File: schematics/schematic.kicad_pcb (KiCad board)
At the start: 2 copper layers, 79.5 x 90 mm, 6 parts, among them Q1 BPW40, U1 L293D, U2 ESP32-S3-DevKitC

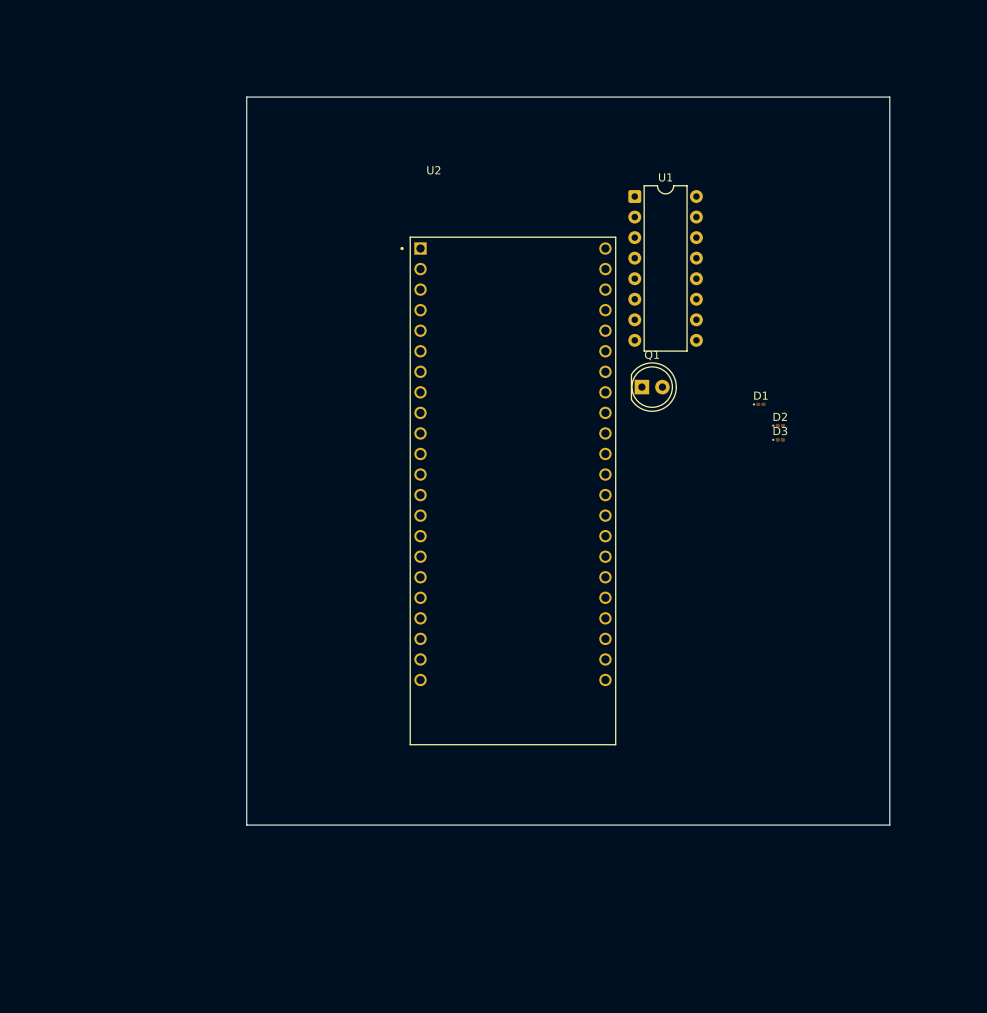
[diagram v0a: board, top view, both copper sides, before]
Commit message: schematic updates
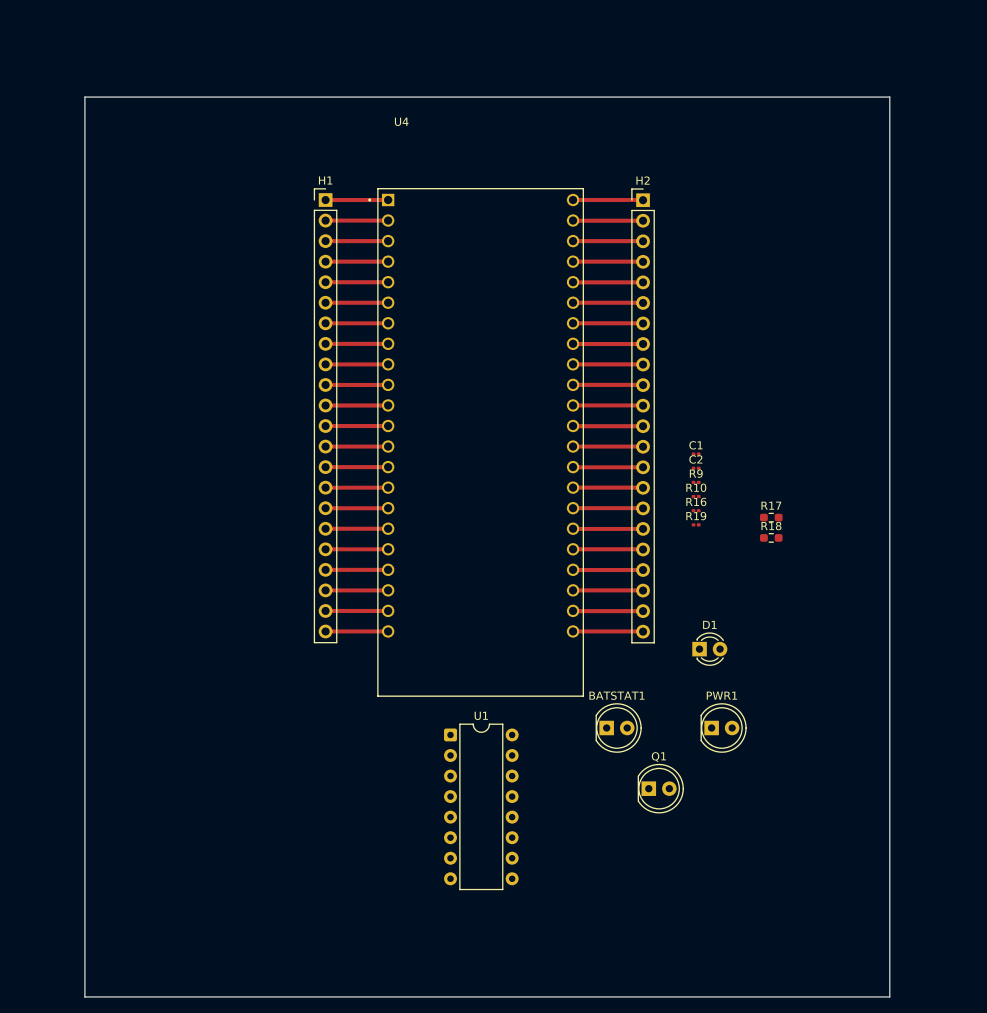
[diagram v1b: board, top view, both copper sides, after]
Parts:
- removed D2: GREEN, LED_SMD:LED_0201_0603Metric
- removed D3: BLUE, LED_SMD:LED_0201_0603Metric
- removed U2: ESP32-S3-DevKitC, footprints_pretty:XCVR_ESP32-S3-DEVKITC-1-N8R2
- added BATSTAT1: LED, LED_THT:LED_D5.0mm, F.Cu at (165.2, 127.5)
- added C1: 0.33 uF, Capacitor_SMD:C_0201_0603Metric, F.Cu at (176.3, 93.6)
- added C2: 0.1 uF, Capacitor_SMD:C_0201_0603Metric, F.Cu at (176.3, 95.4)
- added H1: ~, Connector_PinHeader_2.54mm:PinHeader_1x22_P2.54mm_Vertical, F.Cu at (130.5, 62.2)
- added H2: ~, Connector_PinHeader_2.54mm:PinHeader_1x22_P2.54mm_Vertical, F.Cu at (169.8, 62.2)
- added PWR1: LED, LED_THT:LED_D5.0mm, F.Cu at (178.2, 127.5)
- added R10: 110 kΩ, Resistor_SMD:R_0201_0603Metric, F.Cu at (176.3, 98.9)
- added R16: 1.5 kΩ, Resistor_SMD:R_0201_0603Metric, F.Cu at (176.3, 100.6)
- added R17: 4.7 MΩ, Resistor_SMD:R_0603_1608Metric_Pad0.98x0.95mm_HandSolder, F.Cu at (185.6, 101.5)
- added R18: 2.56 MΩ, Resistor_SMD:R_0603_1608Metric_Pad0.98x0.95mm_HandSolder, F.Cu at (185.6, 104.0)
- added R19: 1.5 kΩ, Resistor_SMD:R_0201_0603Metric, F.Cu at (176.3, 102.4)
- added R9: 110 Ω, Resistor_SMD:R_0201_0603Metric, F.Cu at (176.3, 97.1)
- added U4: ESP32-S3-DEVKITC-1-N8R2, footprints_pretty:XCVR_ESP32-S3-DEVKITC-1-N8R2, F.Cu at (149.7, 92.2)
- D1: value RED -> IR204A; footprint LED_SMD:LED_0201_0603Metric -> LED_THT:LED_D3.0mm_IRBlack
- Q1: footprint LED_THT:LED_D5.0mm_Clear -> LED_THT:LED_D5.0mm
- moved U1 70.4 mm to (145.9, 128.4)
- moved Q1 49.7 mm to (170.5, 135.0)
- moved D1 31.2 mm to (176.7, 117.8)
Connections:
- D1 pad 1: Net-(D1-K) -> Earth
- D1 pad 2: /red_led -> Net-(D1-A)
- Q1 pad 2: /color_sensor -> /J1_15
- U1 pad 10: /right_M1 -> /J3_9
- U1 pad 15: /right_M2 -> /J3_8
- U1 pad 2: /left_M1 -> /J3_19
- U1 pad 7: /left_M2 -> /J1_4
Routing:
- net Earth: track 0.00 -> 33.7 mm
- net +3.3V: track 0.00 -> 15.5 mm
- net /J3_8: track 0.00 -> 8.66 mm
- net /J3_6: track 0.00 -> 8.66 mm
- net /J3_4: track 0.00 -> 8.66 mm
- net /J3_20: track 0.00 -> 8.66 mm
- net /J3_2: track 0.00 -> 8.66 mm
- net /J3_19: track 0.00 -> 8.66 mm
- net /J3_18: track 0.00 -> 8.66 mm
- net /J3_17: track 0.00 -> 8.66 mm
- net /J3_15: track 0.00 -> 8.66 mm
- net /J3_13: track 0.00 -> 8.66 mm
- net /J3_11: track 0.00 -> 8.66 mm
- net /J3_10: track 0.00 -> 8.66 mm
- net /J3_9: track 0.00 -> 8.66 mm
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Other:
- board size 79.5 x 90 mm -> 99.5 x 111.2 mm

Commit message: pcb basically done
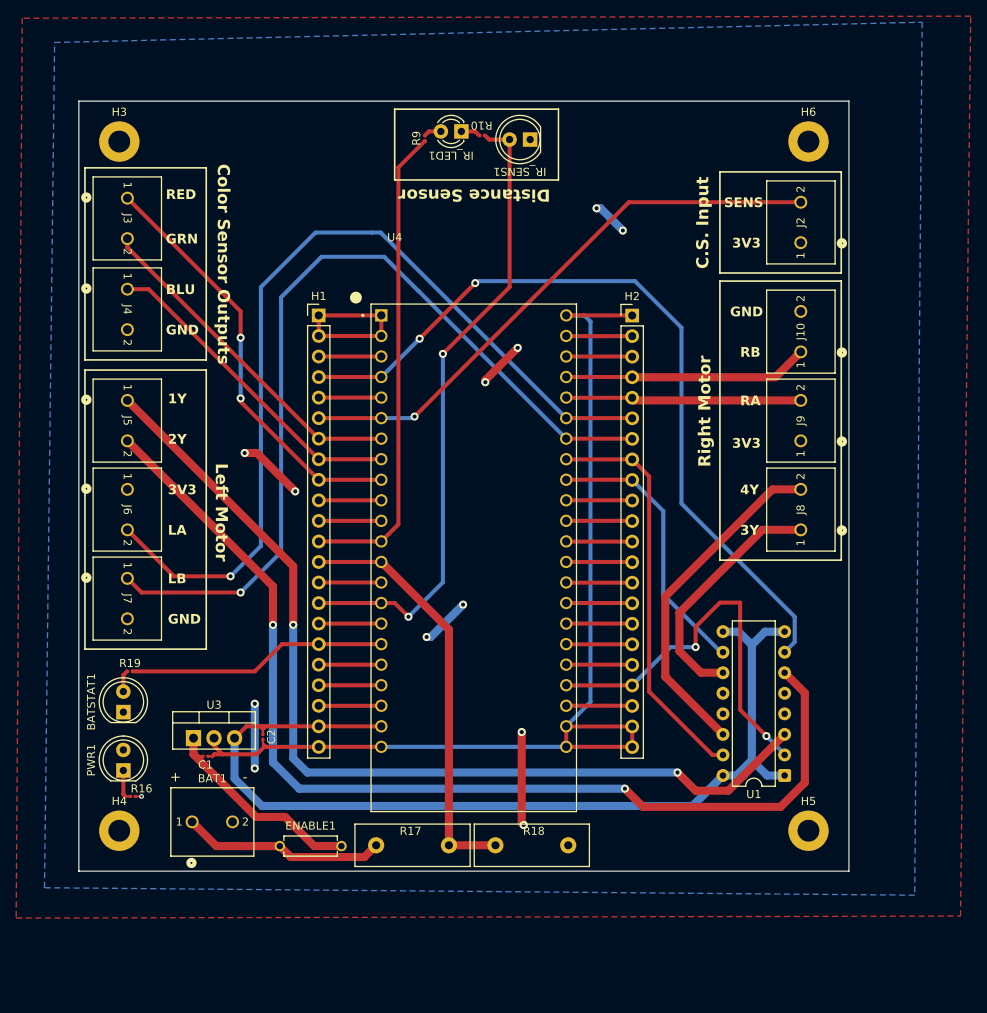
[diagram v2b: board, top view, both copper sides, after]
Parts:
- added BAT1: Conn_01x02, footprints_pretty:CONN2_282836-2_TEC, F.Cu at (119.0, 139.1)
- added ENABLE1: Enable Switch, footprints_pretty:Single Position DIP Switch, F.Cu at (128.7, 142.1)
- added H3: MountingHole, MountingHole:MountingHole_2.7mm_M2.5, F.Cu at (105.0, 55.0)
- added H4: MountingHole, MountingHole:MountingHole_2.7mm_M2.5, F.Cu at (105.0, 140.2)
- added H5: MountingHole, MountingHole:MountingHole_2.7mm_M2.5, F.Cu at (190.2, 140.2)
- added H6: MountingHole, MountingHole:MountingHole_2.7mm_M2.5, F.Cu at (190.2, 55.0)
- added J10: Conn_01x02, footprints_pretty:CONN2_282836-2_TEC, F.Cu at (189.2, 76.0)
- added J2: Conn_01x02, footprints_pretty:CONN2_282836-2_TEC, F.Cu at (189.2, 62.5)
- added J3: Conn_01x02, footprints_pretty:CONN2_282836-2_TEC, F.Cu at (106.0, 67.0)
- added J4: Conn_01x02, footprints_pretty:CONN2_282836-2_TEC, F.Cu at (106.0, 78.2)
- added J5: Conn_01x02, footprints_pretty:CONN2_282836-2_TEC, F.Cu at (106.0, 92.0)
- added J6: Conn_01x02, footprints_pretty:CONN2_282836-2_TEC, F.Cu at (106.0, 103.0)
- added J7: Conn_01x02, footprints_pretty:CONN2_282836-2_TEC, F.Cu at (106.0, 114.0)
- added J8: Conn_01x02, footprints_pretty:CONN2_282836-2_TEC, F.Cu at (189.2, 98.0)
- added J9: Conn_01x02, footprints_pretty:CONN2_282836-2_TEC, F.Cu at (189.2, 87.0)
- added U3: L7805, Package_TO_SOT_THT:TO-220-3_Vertical, F.Cu at (114.2, 128.8)
- R17, R18: footprint Resistor_SMD:R_0603_1608Metric_Pad0.98x0.95mm_HandSolder -> Resistor_THT:R_Box_L14.0mm_W5.0mm_P9.00mm
- moved IR_SENS1 81.6 mm to (155.8, 54.8), turned to 180 degrees
- moved R16 78.1 mm to (106.7, 136.0)
- moved PWR1 72.9 mm to (105.5, 132.8), turned to 90 degrees
- moved R19 72.3 mm to (106.3, 120.5), turned to 180 degrees
- moved C1 71.2 mm to (115.7, 131.0), turned to 180 degrees
- moved IR_LED1 70.4 mm to (147.3, 53.8), turned to 180 degrees
- moved C2 63.0 mm to (122.8, 128.6), turned to -90 degrees
- moved BATSTAT1 59.8 mm to (105.5, 125.5), turned to 90 degrees
- moved R17 56.8 mm to (145.8, 142.0), turned to 180 degrees
- moved R9 54.2 mm to (142.8, 54.6), turned to 90 degrees
- moved R10 51.9 mm to (149.9, 54.2)
- moved R18 45.5 mm to (160.5, 142.0), turned to 180 degrees
- moved U1 41.6 mm to (187.2, 133.4), turned to 180 degrees
- moved H2 14.3 mm to (168.4, 76.5)
- moved H1 14.3 mm to (129.7, 76.5)
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- renumbered D1 to IR_LED1, Q1 to IR_SENS1
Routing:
- net Net-(J5-Pin_2): track 0.00 -> 131.1 mm, vias 0 -> 2
- net Earth: track 33.7 -> 153.2 mm, vias 0 -> 5
- net Net-(J5-Pin_1): track 0.00 -> 118.0 mm, vias 0 -> 2
- net +5V: track 7.74 -> 122.1 mm
- net /J3_6: track 8.66 -> 111.1 mm, vias 0 -> 1
- net /J3_7: track 8.66 -> 108.6 mm, vias 0 -> 1
- net /J1_4: track 7.74 -> 98.6 mm, vias 0 -> 2
- net /J1_15: track 7.74 -> 79.2 mm, vias 0 -> 2
- net /J1_6: track 7.74 -> 70.7 mm, vias 0 -> 1
- net /J1_12: track 7.74 -> 59.5 mm
- net /J1_9: track 7.74 -> 52.4 mm, vias 0 -> 2
- net /J1_13: track 7.74 -> 52.0 mm
- net Net-(J8-Pin_2): track 0.00 -> 42.2 mm
- net /J3_8: track 8.66 -> 50.6 mm
- net /J3_19: track 8.66 -> 48.8 mm, vias 0 -> 2
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- added copper zone on F.Cu, net +3.3V
- added copper zone on B.Cu, net Earth
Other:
- board size 99.5 x 111.2 mm -> 95.2 x 95.2 mm
- board text added: "+"
- board text added: "-"
- board text added: "1Y"
- board text added: "2Y"
- board text added: "3V3"
- board text added: "3Y"
- board text added: "4Y"
- board text added: "BLU"
- board text added: "C.S. Input"
- board text added: "Color Sensor Outputs"
- board text added: "Distance Sensor"
- board text added: "GND"
- board text added: "GRN"
- board text added: "LA"
- board text added: "LB"
- board text added: "Left Motor"
- board text added: "RA"
- board text added: "RB"
- board text added: "RED"
- board text added: "Right Motor"
- board text added: "SENS"
